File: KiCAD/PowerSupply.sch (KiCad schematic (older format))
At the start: 13 parts, among them J2 USB_Micro_B, J3 Binder 709 Female Panel Mount, Q1 3.7A, 30V, U2 AP2112K-3.3, U3 LM1117

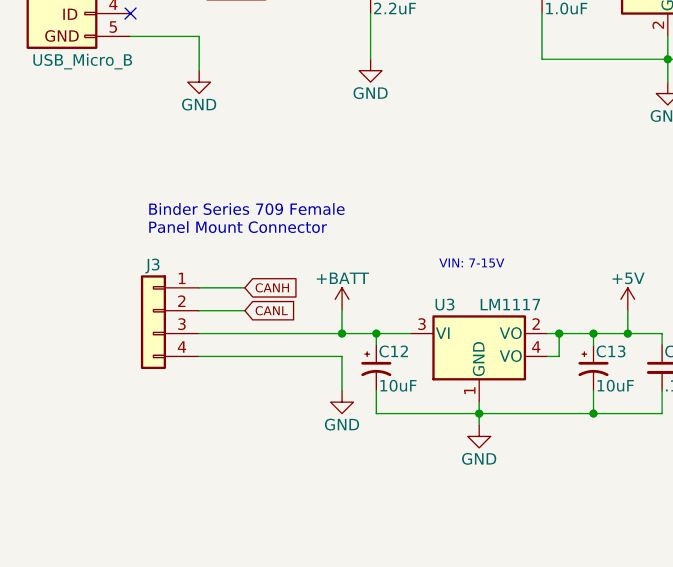
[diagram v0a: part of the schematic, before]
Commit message: Redoing layout
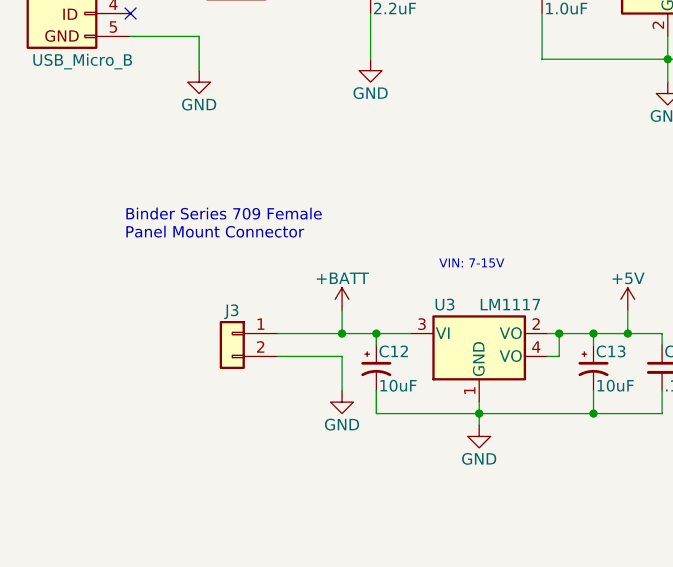
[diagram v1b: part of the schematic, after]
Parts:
- removed J3: Binder 709 Female Panel Mount, Pin_Headers:Pin_Header_Straight_1x04_Pitch2.54mm, symbol Conn_01x04
- added J3: Battery Headers, Pin_Headers:Pin_Header_Straight_1x02_Pitch2.54mm, symbol Conn_01x02
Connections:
- net +BATT: now also J3.1 (Pin_1)
- net GND: now also J3.2 (Pin_2)
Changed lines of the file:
@@
 	1    0    0    -1
 $EndComp
-$Comp
-L Conn_01x04 J3
-U 1 1 5C661C12
-P 4500 4600
-F 0 "J3" H 4500 4800 50  0000 C CNN
-F 1 "Binder 709 Female Panel Mount" H 4500 4300 50  0001 C CNN
-F 2 "Pin_Headers:Pin_Header_Straight_1x04_Pitch2.54mm" H 4500 4600 50  0001 C CNN
-F 3 "" H 4500 4600 50  0001 C CNN
-	1    4500 4600
-	-1   0    0    -1
-$EndComp
-Text GLabel 4900 4500 2    39   Input ~ 0
-CANH
-Text GLabel 4900 4600 2    39   Input ~ 0
-CANL
-Text Notes 4475 4275 0    49   ~ 0
+Text Notes 4375 4295 0    49   ~ 0
 Binder Series 709 Female \nPanel Mount Connector
 $Comp
@@
 Wire Wire Line
 	5925 5100 5925 5000
-Wire Wire Line
-	4700 4700 5625 4700
 Wire Wire Line
 	6225 4800 6275 4800
@@
 	4400 3100 4700 3100
 Wire Wire Line
-	4700 4500 4900 4500
-Wire Wire Line
-	4700 4600 4900 4600
-Wire Wire Line
-	5325 4800 4700 4800
-Wire Wire Line
 	4675 2900 4675 3000
 Connection ~ 4675 3000
+$Comp
+L Conn_01x02 J3
+U 1 1 5C9D06F2
+P 4845 4700
+F 0 "J3" H 4845 4800 50  0000 C CNN
+F 1 "Battery Headers" H 4845 4500 50  0001 C CNN
+F 2 "Pin_Headers:Pin_Header_Straight_1x02_Pitch2.54mm" H 4845 4700 50  0001 C CNN
+F 3 "" H 4845 4700 50  0001 C CNN
+	1    4845 4700
+	-1   0    0    -1
+$EndComp
+Wire Wire Line
+	5045 4700 5625 4700
+Wire Wire Line
+	5325 4800 5045 4800
 $EndSCHEMATC
